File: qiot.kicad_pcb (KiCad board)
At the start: 4 copper layers, 599 parts, among them IC1 MC33926AES, J1 Conn_01x03, J10 CELLS1, J11 Conn_01x03, J12 EN, J13 Conn_01x03, J14 Barrel_Jack, J15 TYPE-C-31-M-12, J16 Conn_01x04, J17 Conn_01x03, J18 Conn_01x03, J19 Conn_01x03, J2 Conn_01x05, J20 Conn_01x05, J21 PWRSWITCH, J22 Conn_01x02, J23 PGOOD, J24 68000-202HLF, J25 Conn_01x03_Pin, J26 Conn_01x03, J27 Conn_01x02, J28 Conn_01x02, J29 Conn_01x02, J3 TE_4-1734592-0, J30 Conn_01x04, J31 TYPE-C-31-M-12, J32 Conn_01x03, J33 EnUSB, J34 BAMBANG_CONNECTOR, J35 TE_4-1734592-0, J36 Conn_02x10_Odd_Even, J37 RJ45_Hanrun_HR911105A_Horizon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, J38 RJHSE5380, J39 Conn_01x03, J4 Conn_02x03_Odd_Even, J40 Conn_01x02, J41 Conn_01x02, J42 Conn_01x02, J5 BATT1_jmp, J6 BATT2_jmp, J7 Conn_01x03, J8 Conn_01x03, J9 CELLS1, Q1 PMBT2222A, Q10 PSMN4R2-30MLD, Q11 PSMN4R2-30MLD, Q12 PSMN4R2-30MLD, Q13 PSMN4R2-30MLD, Q14 PSMN4R2-30MLD, Q15 PMBT2222A, Q16 PMBT2222A, Q17 PMBT2222A, Q18 PMBT2222A, Q19 PMBT2222A, Q2 PMBT2222A, Q20 PMBT2222A, Q21 PMBT2222A, Q22 BC817, Q23 PSMN4R2-30MLD, Q24 MMBT3904WT1G, Q3 IRLZ44NSTRL(UMW), Q4 IRLZ44NSTRL(UMW), Q5 PMBT2222A, Q6 2N7002, Q7 BSS223PW, Q8 IRLZ44NSTRL(UMW), Q9 IRLZ44NSTRL(UMW), U1 MIMXRT1011DAE5A, U10 MC34GD3000EP, U11 TLV62130, U12 TLV62130, U13 FC41D, U14 PCA9539PW_118, U15 MIMXRT1062DVL6B, U16 UM803RS, U17 KSZ8081RNBCA-TR, U18 SRV05-4, U19 MAX3232, U2 UM803RS, U20 IS42S16160J-6BLI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

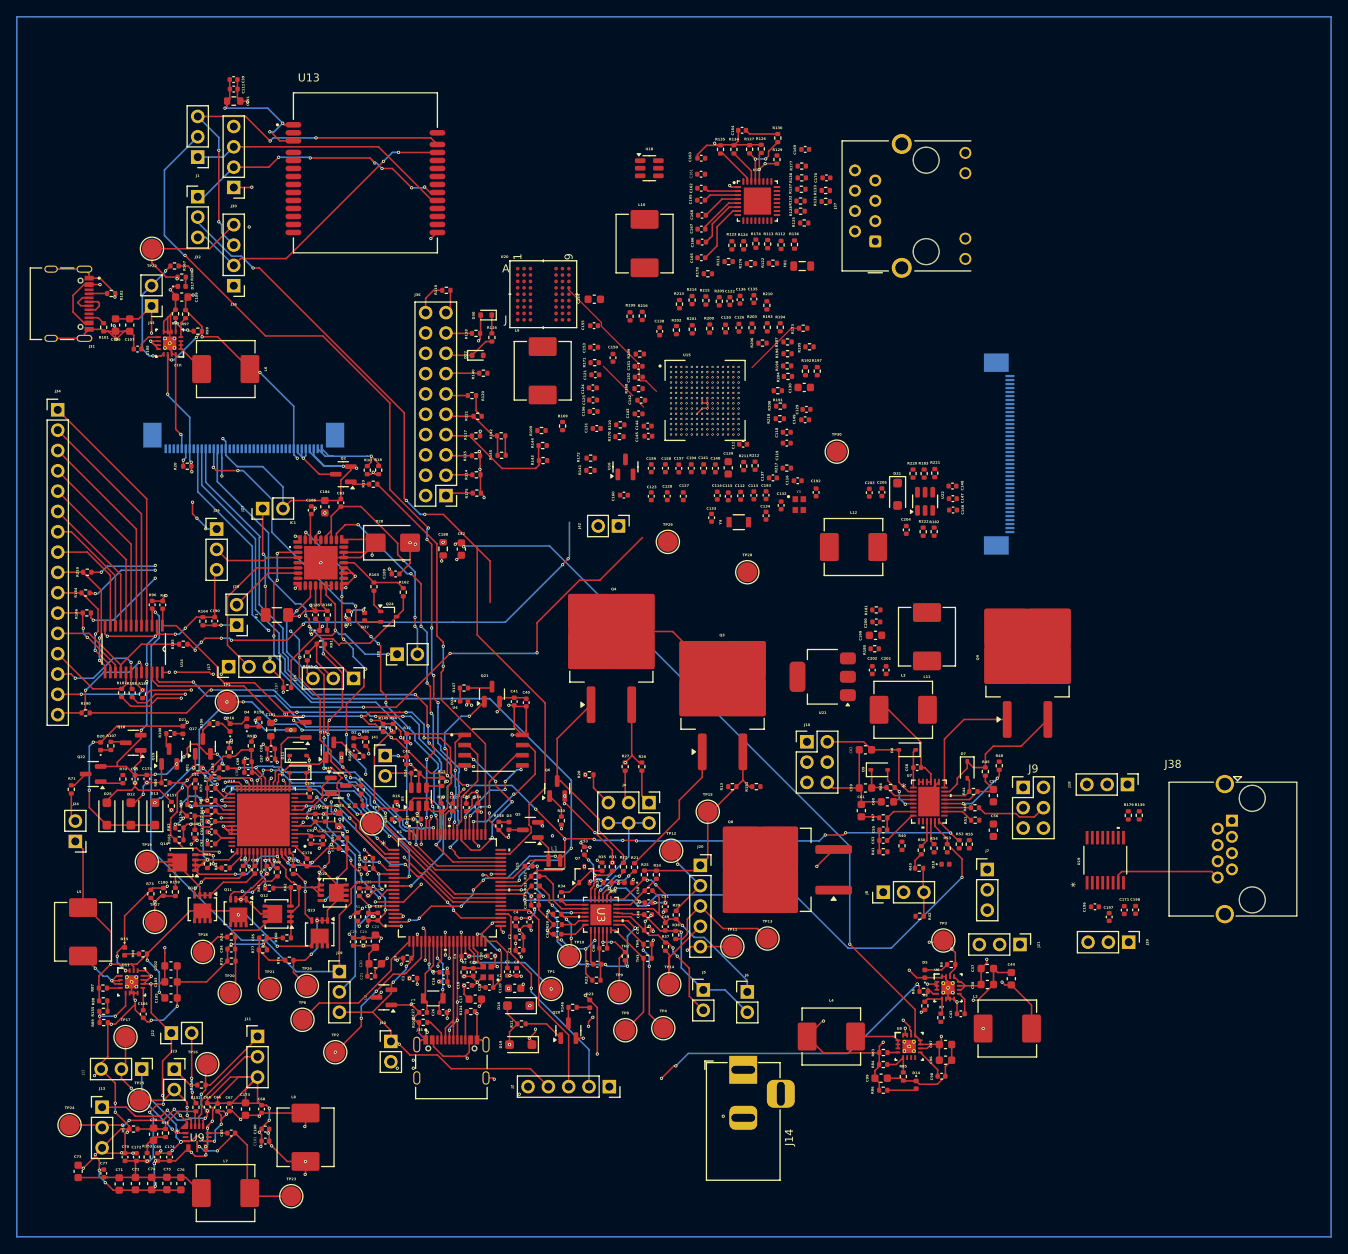
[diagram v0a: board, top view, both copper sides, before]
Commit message: mera
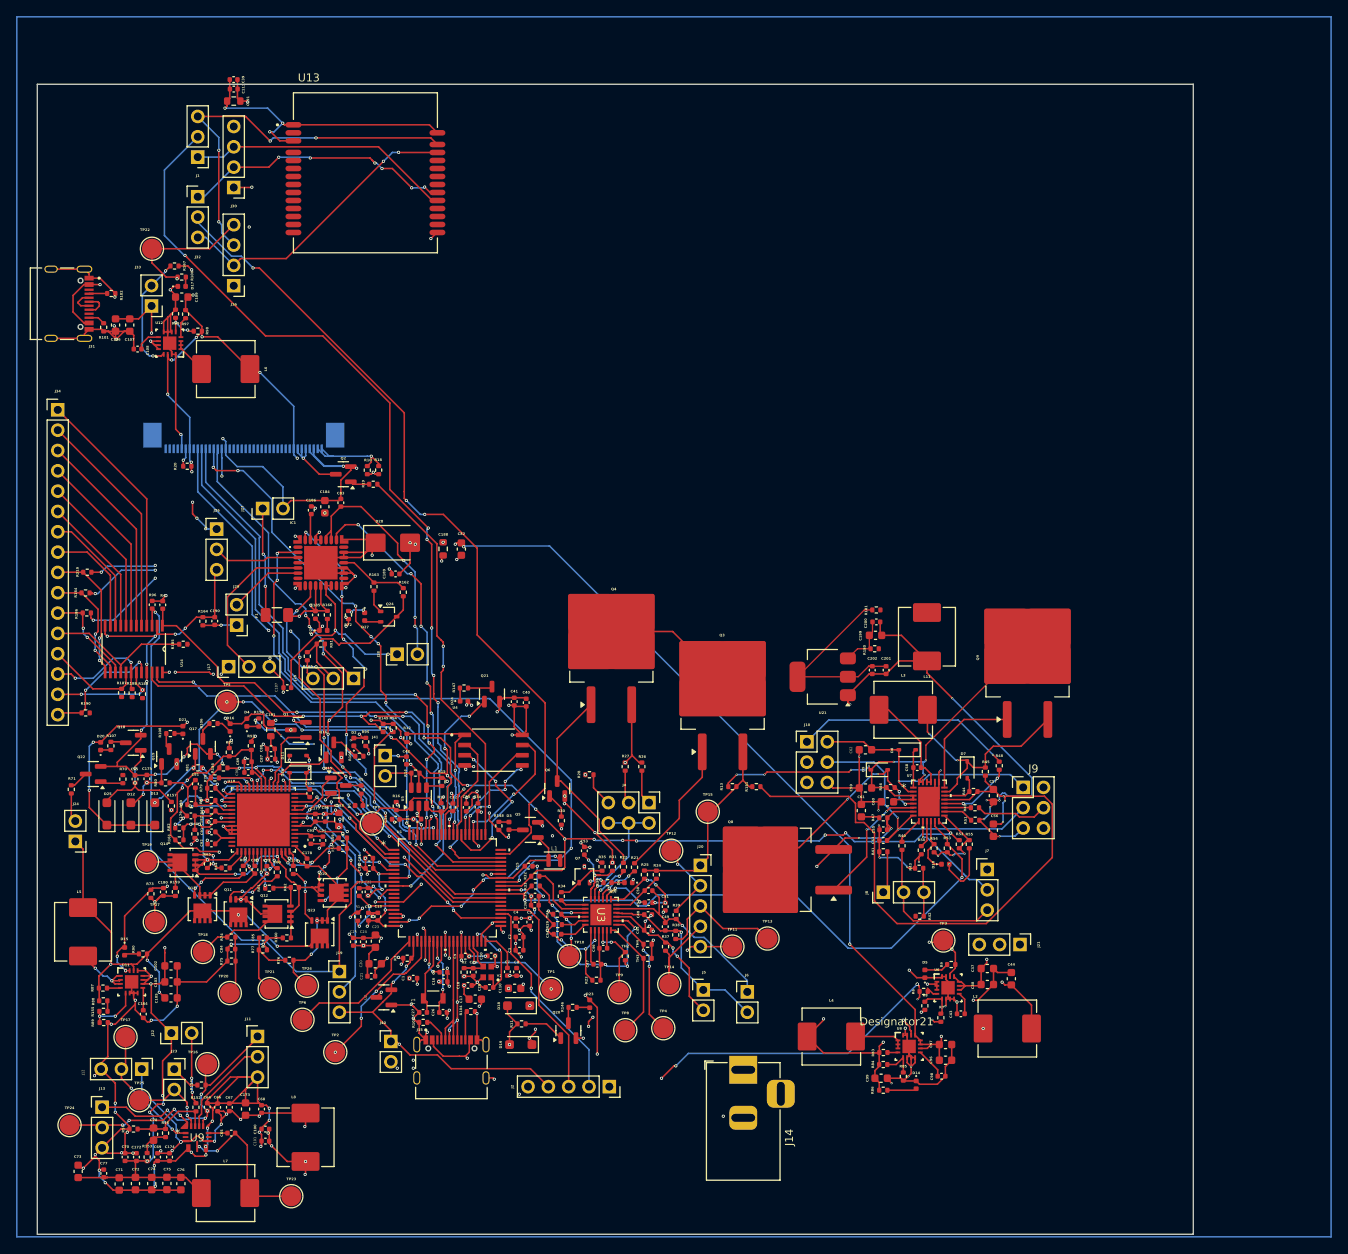
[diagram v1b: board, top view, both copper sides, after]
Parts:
- removed C112, C114, C116, C117, C118, C120, C122, C123, C124, C125, C126, C127, C128, C129, C153, C155, C156, C158, C159, C193: 0.22uF, Capacitor_SMD:C_0402_1005Metric
- removed C113, C115, C121, C135, C143, C144, C147, C152, C161, C204: 4.7uF, Capacitor_SMD:C_0402_1005Metric
- removed C119, C141, C194: 1.0uF, Capacitor_SMD:C_0402_1005Metric
- removed C130: 22uF, Capacitor_SMD:C_0603_1608Metric
- removed C131, C136, C137, C138, C140, C142, C145, C146, C148, C149, C150, C151, C160, C162, C164, C169, C170, C171, C195, C196, C197, C198, C203: 0.1uF, Capacitor_SMD:C_0402_1005Metric
- removed C132, C192: 4.7pF, Capacitor_SMD:C_0402_1005Metric
- removed C133, C134, C165, C166, C167, C168: 10pF, Capacitor_SMD:C_0402_1005Metric
- removed C139: 10uF, Capacitor_SMD:C_0603_1608Metric
- removed C154: 33uF, Capacitor_SMD:C_0603_1608Metric
- removed C157: 0.47uF, Capacitor_SMD:C_0402_1005Metric
- removed C163, C205: 2.2uF, Capacitor_SMD:C_0402_1005Metric
- removed D22, D30: RB521S30, Diode_SMD:D_SOD-523
- removed D31: PMEG3020EH, Diode_SMD:D_SOD-123F
- removed FB1: BLM21PG221SN1D, Inductor_SMD:L_0805_2012Metric
- removed J18, J39: Conn_01x03, Connector_PinHeader_2.54mm:PinHeader_1x03_P2.54mm_Vertical
- removed J35: TE_4-1734592-0, footprints:TE_4-1734592-0
- removed J36: Conn_02x10_Odd_Even, Connector_PinHeader_2.54mm:PinHeader_2x10_P2.54mm_Vertical
- removed J37: RJ45_Hanrun_HR911105A_Horizontal, Connector_RJ:RJ45_Hanrun_HR911105A_Horizontal
- removed J38: RJHSE5380, Connector_RJ:RJ45_Amphenol_RJHSE5380
- removed J42: Conn_01x02, Connector_PinHeader_2.54mm:PinHeader_1x02_P2.54mm_Vertical
- removed L10: L_Iron, Inductor_SMD:L_APV_APH0620
- removed L12: 10uH, Inductor_SMD:L_APV_APH0620
- removed L9: 4.7uH, Inductor_SMD:L_APV_APH0620
- removed R109, R140, R141, R142, R143, R144, R145, R168, R172, R173, R178, R183, R220: 0, Resistor_SMD:R_0402_1005Metric
- removed R110, R114, R115, R116, R117, R118, R119, R120, R121, R170, R191, R193, R196, R198, R207, R208, R209, R210, R213, R214, R215, R216, R217, R218: 10K, Resistor_SMD:R_0402_1005Metric
- removed R111, R112, R113, R126, R127, R128, R132, R134, R135, R136, R138, R139, R174, R176, R177, R179, R192, R194, R195, R197, R199, R200, R201, R202, R203, R204, R205, R206, R211, R212: 1K, Resistor_SMD:R_0402_1005Metric
- removed R122: 6.49K, Resistor_SMD:R_0402_1005Metric
- removed R123, R124, R125, R129, R130, R131, R133, R137: 4.7K, Resistor_SMD:R_0402_1005Metric
- removed R169: 1.5K, Resistor_SMD:R_0402_1005Metric
- removed R171: 30K, Resistor_SMD:R_0402_1005Metric
- removed R175: 100, Resistor_SMD:R_0402_1005Metric
- removed R182, R222: 10, Resistor_SMD:R_0402_1005Metric
- removed R221: 100k, Resistor_SMD:R_0402_1005Metric
- removed TP28, TP29, TP30: TestPoint, TestPoint:TestPoint_Pad_D2.5mm
- removed U15: MIMXRT1062DVL6B, footprints:BGA196C65P14X14_1000X1000X152N
- removed U16: UM803RS, Package_TO_SOT_SMD:SOT-23
- removed U17: KSZ8081RNBCA-TR, footprints:QFN50P500X500X100-33N
- removed U18: SRV05-4, Package_TO_SOT_SMD:SOT-23-6
- removed U19: MAX3232, footprints:PW16_TEX
- removed U20: IS42S16160J-6BLI, footprints:TFBGA-54_8X8_ISI
- removed U22: UM1663S, Package_TO_SOT_SMD:SOT-23-6
- removed Y3: 24MHZ, footprints:OSC_XRCGB24M000F2P29R0
- removed Y4: 32.768KHZ, footprints:CRYSTAL_FC-135 32.7680KA-AG3_EPS
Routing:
- net SYSN: track 965.1 -> 1091.3 mm, vias 187 -> 177
- net GPIO_AD_B1_07: track 82.2 -> 0.00 mm, vias 5 -> 0
- net BATSENS_CHG: track 8.77 -> 81.7 mm, vias 0 -> 3
- net GPIO_AD_B1_03: track 57.9 -> 0.23 mm, vias 8 -> 0
- net VOUT_BATCHG: track 11.1 -> 57.7 mm, vias 0 -> 7
- net Net-(J10-Pin_4): track 4.57 -> 38.7 mm, vias 0 -> 2
- net DCDC_3V3: track 32.2 -> 0.00 mm, vias 11 -> 0
- net Net-(J10-Pin_1): track 5.08 -> 32.5 mm, vias 0 -> 2
- net VDD_1V8: track 0.00 -> 24.5 mm
- net 3P3V: track 484.6 -> 505.9 mm, vias 77 -> 82
- net Net-(J7-Pin_3): track 0.00 -> 19.3 mm
- net SEMC_D5: track 17.9 -> 0.00 mm, vias 1 -> 0
- net Net-(D9-A): track 6.30 -> 23.8 mm, vias 2 -> 4
- net INTVcc: track 15.7 -> 32.3 mm, vias 0 -> 1
- net Net-(Q8-G): track 0.00 -> 16.3 mm, vias 0 -> 2
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- added copper zone on In2.Cu, net /07_dcdcConv/VSUP
- added copper zone on In1.Cu, net SYSN
- added copper zone on In2.Cu, net VCC_12V
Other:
- board outline added: 144.5 x 143.8 mm
